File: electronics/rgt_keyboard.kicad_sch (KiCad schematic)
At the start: 61 parts, among them J5 Conn_01x05_Female, J6 Conn_01x05_Male, SW30 SW_SPST, SW31 SW_SPST, SW32 SW_SPST, SW33 SW_SPST, SW34 SW_SPST, SW35 SW_SPST, SW36 SW_SPST, SW37 SW_SPST, SW38 SW_SPST, SW39 SW_SPST, SW40 SW_SPST, SW41 SW_SPST, SW42 SW_SPST, SW43 SW_SPST, SW44 SW_SPST, SW45 SW_SPST, SW46 SW_SPST, SW47 SW_SPST, SW48 SW_SPST, SW49 SW_SPST, SW50 SW_SPST, SW51 SW_SPST, SW52 SW_SPST, SW53 SW_SPST, SW54 SW_SPST, SW55 SW_SPST, SW56 SW_SPST, SW57 SW_SPST, SW58 SW_SPST, U3 PCA9675PW

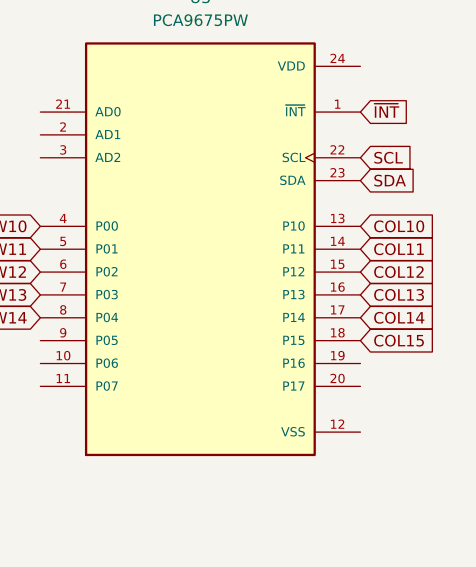
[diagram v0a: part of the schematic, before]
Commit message: finish matrix
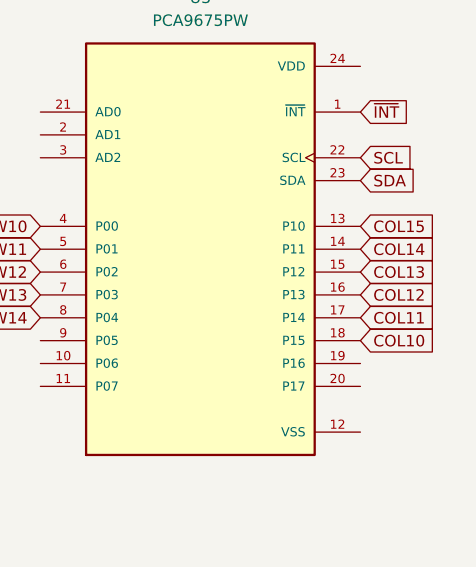
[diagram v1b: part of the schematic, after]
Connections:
- net COL10: now also U3.18 (P15); no longer U3.13 (P10)
- net COL11: now also U3.17 (P14); no longer U3.14 (P11)
- net COL12: now also U3.16 (P13); no longer U3.15 (P12)
- net COL13: now also U3.15 (P12); no longer U3.16 (P13)
- net COL14: now also U3.14 (P11); no longer U3.17 (P14)
- net COL15: now also U3.13 (P10); no longer U3.18 (P15)
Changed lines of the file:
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@@
     (stroke (width 0) (type default) (color 0 0 0 0))
   )
+  (global_label "COL15" (shape input) (at 246.38 46.99 0) (fields_autoplaced)
+    (effects (font (size 1.27 1.27)) (justify left))
+    (property "Intersheet References" "${INTERSHEET_REFS}" (id 0) (at 254.8407 46.9106 0)
+      (effects (font (size 1.27 1.27)) (justify left) hide)
+    )
+  )
   (global_label "~{INT}" (shape input) (at 240.03 124.46 0) (fields_autoplaced)
     (effects (font (size 1.27 1.27)) (justify left))
@@
     )
   )
-  (global_label "COL10" (shape input) (at 246.38 46.99 0) (fields_autoplaced)
-    (effects (font (size 1.27 1.27)) (justify left))
-    (property "Intersheet References" "${INTERSHEET_REFS}" (id 0) (at 254.8407 47.0694 0)
-      (effects (font (size 1.27 1.27)) (justify left) hide)
-    )
-  )
   (global_label "ROW14" (shape input) (at 38.1 156.21 180) (fields_autoplaced)
     (effects (font (size 1.27 1.27)) (justify right))
@@
     )
   )
+  (global_label "COL12" (shape input) (at 246.38 54.61 0) (fields_autoplaced)
+    (effects (font (size 1.27 1.27)) (justify left))
+    (property "Intersheet References" "${INTERSHEET_REFS}" (id 0) (at 254.8407 54.5306 0)
+      (effects (font (size 1.27 1.27)) (justify left) hide)
+    )
+  )
   (global_label "COL15" (shape input) (at 149.86 83.82 180) (fields_autoplaced)
     (effects (font (size 1.27 1.27)) (justify right))
@@
     )
   )
-  (global_label "COL14" (shape input) (at 246.38 57.15 0) (fields_autoplaced)
-    (effects (font (size 1.27 1.27)) (justify left))
-    (property "Intersheet References" "${INTERSHEET_REFS}" (id 0) (at 254.8407 57.2294 0)
-      (effects (font (size 1.27 1.27)) (justify left) hide)
-    )
-  )
   (global_label "ROW10" (shape input) (at 139.7 92.71 180) (fields_autoplaced)
     (effects (font (size 1.27 1.27)) (justify right))
@@
     )
   )
+  (global_label "COL14" (shape input) (at 246.38 49.53 0) (fields_autoplaced)
+    (effects (font (size 1.27 1.27)) (justify left))
+    (property "Intersheet References" "${INTERSHEET_REFS}" (id 0) (at 254.8407 49.4506 0)
+      (effects (font (size 1.27 1.27)) (justify left) hide)
+    )
+  )
   (global_label "ROW12" (shape input) (at 78.74 124.46 180) (fields_autoplaced)
     (effects (font (size 1.27 1.27)) (justify right))
@@
     )
   )
-  (global_label "COL13" (shape input) (at 246.38 54.61 0) (fields_autoplaced)
-    (effects (font (size 1.27 1.27)) (justify left))
-    (property "Intersheet References" "${INTERSHEET_REFS}" (id 0) (at 254.8407 54.6894 0)
-      (effects (font (size 1.27 1.27)) (justify left) hide)
-    )
-  )
   (global_label "~{INT}" (shape input) (at 246.38 34.29 0) (fields_autoplaced)
     (effects (font (size 1.27 1.27)) (justify left))
@@
     )
   )
+  (global_label "COL11" (shape input) (at 246.38 57.15 0) (fields_autoplaced)
+    (effects (font (size 1.27 1.27)) (justify left))
+    (property "Intersheet References" "${INTERSHEET_REFS}" (id 0) (at 254.8407 57.0706 0)
+      (effects (font (size 1.27 1.27)) (justify left) hide)
+    )
+  )
   (global_label "ROW11" (shape input) (at 139.7 107.95 180) (fields_autoplaced)
     (effects (font (size 1.27 1.27)) (justify right))
@@
     )
   )
-  (global_label "COL12" (shape input) (at 246.38 52.07 0) (fields_autoplaced)
-    (effects (font (size 1.27 1.27)) (justify left))
-    (property "Intersheet References" "${INTERSHEET_REFS}" (id 0) (at 254.8407 52.1494 0)
-      (effects (font (size 1.27 1.27)) (justify left) hide)
-    )
-  )
   (global_label "ROW11" (shape input) (at 210.82 49.53 180) (fields_autoplaced)
     (effects (font (size 1.27 1.27)) (justify right))
@@
     )
   )
-  (global_label "COL15" (shape input) (at 246.38 59.69 0) (fields_autoplaced)
-    (effects (font (size 1.27 1.27)) (justify left))
-    (property "Intersheet References" "${INTERSHEET_REFS}" (id 0) (at 254.8407 59.7694 0)
-      (effects (font (size 1.27 1.27)) (justify left) hide)
-    )
-  )
   (global_label "ROW10" (shape input) (at 38.1 92.71 180) (fields_autoplaced)
     (effects (font (size 1.27 1.27)) (justify right))
@@
     )
   )
-  (global_label "COL11" (shape input) (at 246.38 49.53 0) (fields_autoplaced)
-    (effects (font (size 1.27 1.27)) (justify left))
-    (property "Intersheet References" "${INTERSHEET_REFS}" (id 0) (at 254.8407 49.6094 0)
-      (effects (font (size 1.27 1.27)) (justify left) hide)
-    )
-  )
   (global_label "ROW14" (shape input) (at 99.06 156.21 180) (fields_autoplaced)
     (effects (font (size 1.27 1.27)) (justify right))
@@
     )
   )
+  (global_label "COL10" (shape input) (at 246.38 59.69 0) (fields_autoplaced)
+    (effects (font (size 1.27 1.27)) (justify left))
+    (property "Intersheet References" "${INTERSHEET_REFS}" (id 0) (at 254.8407 59.6106 0)
+      (effects (font (size 1.27 1.27)) (justify left) hide)
+    )
+  )
   (global_label "ROW14" (shape input) (at 119.38 156.21 180) (fields_autoplaced)
     (effects (font (size 1.27 1.27)) (justify right))
@@
     )
   )
+  (global_label "COL13" (shape input) (at 246.38 52.07 0) (fields_autoplaced)
+    (effects (font (size 1.27 1.27)) (justify left))
+    (property "Intersheet References" "${INTERSHEET_REFS}" (id 0) (at 254.8407 51.9906 0)
+      (effects (font (size 1.27 1.27)) (justify left) hide)
+    )
+  )
